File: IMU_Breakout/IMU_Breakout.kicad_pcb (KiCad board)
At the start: 2 copper layers, 12 x 11.2 mm, 4 parts, among them J1 Conn_01x04_Socket, U1 LSM6DSL

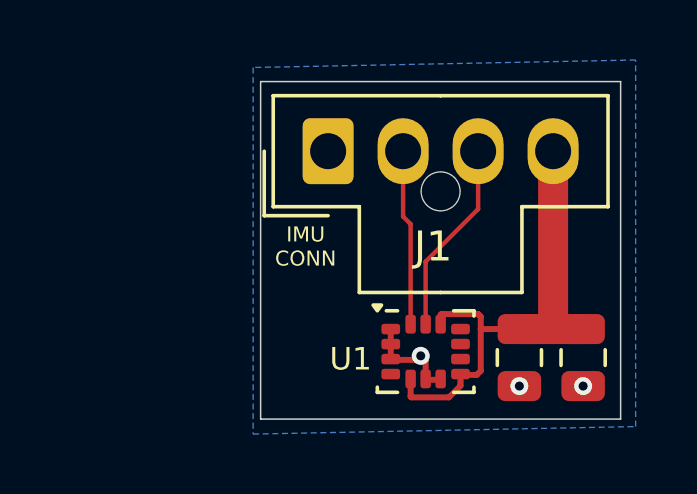
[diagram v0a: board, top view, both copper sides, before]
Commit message: made bom
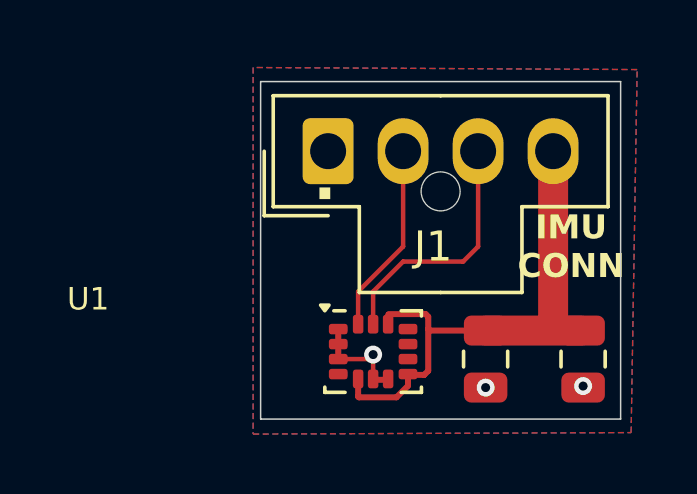
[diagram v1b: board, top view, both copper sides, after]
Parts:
- moved U1 1.75 mm to (146.0, 93.5)
- moved C1 1.13 mm to (149.8, 93.8)
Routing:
- net /IMU_I2C_SCL: track 6.74 -> 8.39 mm
- net +1V8: track 16.5 -> 18.0 mm
- added copper zone on F.Cu, net GND
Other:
- board text added: "."
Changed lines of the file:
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@@
 	(footprint "Capacitor_SMD:C_0805_2012Metric"
 		(layer "F.Cu")
-		(at 150.875 93.7 -90)
+		(at 149.75 93.75 -90)
 		(descr "Capacitor SMD 0805 (2012 Metric), square (rectangular) end terminal, IPC_7351 nominal, (Body size source: IPC-SM-782 page 76, https://www.pcb-3d.com/wordpress/wp-content/uploads/ipc-sm-782a_amendment_1_and_2.pdf, https://docs.google.com/spreadsheets/d/1BsfQQcO9C6DZCsRaXUlFlo91Tg2WpOkGARC1WS5S8t0/edit?usp=sharing), generated with kicad-footprint-generator")
 		(tags "capacitor")
@@
 	(footprint "Capacitor_SMD:C_0805_2012Metric"
 		(layer "F.Cu")
-		(at 153 93.7 -90)
+		(at 153 93.75 -90)
 		(descr "Capacitor SMD 0805 (2012 Metric), square (rectangular) end terminal, IPC_7351 nominal, (Body size source: IPC-SM-782 page 76, https://www.pcb-3d.com/wordpress/wp-content/uploads/ipc-sm-782a_amendment_1_and_2.pdf, https://docs.google.com/spreadsheets/d/1BsfQQcO9C6DZCsRaXUlFlo91Tg2WpOkGARC1WS5S8t0/edit?usp=sharing), generated with kicad-footprint-generator")
 		(tags "capacitor")
@@
 	(footprint "Package_LGA:LGA-14_3x2.5mm_P0.5mm_LayoutBorder3x4y"
 		(layer "F.Cu")
-		(at 147.75 93.5)
+		(at 146 93.5)
 		(descr "LGA, 14 Pin (https://www.st.com/resource/en/datasheet/lsm6ds3tr-c.pdf), generated with kicad-footprint-generator ipc_noLead_generator.py")
 		(tags "LGA NoLead")
 		(property "Reference" "U1"
-			(at -2.5 0.25 0)
+			(at -9.5 -1.75 0)
 			(layer "F.SilkS")
 			(effects
@@
 	)
 	(gr_text "IMU\nCONN"
-		(at 143.75 90 0)
+		(at 152.6 90 0)
 		(layer "F.SilkS")
 		(effects
 			(font
-				(size 0.5 0.5)
-				(thickness 0.125)
-			)
-		)
-	)
-	(segment
-		(start 147.75 92.5875)
-		(end 147.75 90.5)
+				(size 0.8 0.8)
+				(thickness 0.15)
+				(bold yes)
+			)
+		)
+	)
+	(gr_text "."
+		(at 144 88.6 0)
+		(layer "F.SilkS")
+		(effects
+			(font
+				(size 1.5 1.5)
+				(thickness 0.3)
+				(bold yes)
+			)
+			(justify left bottom)
+		)
+	)
+	(segment
+		(start 146 92.5875)
+		(end 146 91.5)
 		(width 0.15)
 		(layer "F.Cu")
@@
 	)
 	(segment
-		(start 149.5 88.75)
-		(end 149.5 86.57)
+		(start 149.5 90)
+		(end 149 90.5)
 		(width 0.15)
 		(layer "F.Cu")
@@
 	)
 	(segment
-		(start 147.75 90.5)
-		(end 149.5 88.75)
+		(start 149.5 86.82)
+		(end 149.5 90)
 		(width 0.15)
 		(layer "F.Cu")
@@
 	)
 	(segment
-		(start 147.25 89.25)
-		(end 147 89)
+		(start 146 91.5)
+		(end 147 90.5)
 		(width 0.15)
 		(layer "F.Cu")
+		(net 1)
+	)
+	(segment
+		(start 147 90.5)
+		(end 149 90.5)
+		(width 0.15)
+		(layer "F.Cu")
+		(net 1)
+	)
+	(segment
+		(start 147 90)
+		(end 147 86.82)
+		(width 0.15)
+		(layer "F.Cu")
 		(net 2)
 	)
 	(segment
-		(start 147.25 92.5875)
-		(end 147.25 89.25)
+		(start 145.5 92.5875)
+		(end 145.5 91.5)
 		(width 0.15)
 		(layer "F.Cu")
@@
 	)
 	(segment
-		(start 147 89)
-		(end 147 86.57)
+		(start 145.5 91.5)
+		(end 147 90)
 		(width 0.15)
 		(layer "F.Cu")
@@
 	)
 	(segment
-		(start 146.5875 93.7775)
-		(end 147.4525 93.7775)
+		(start 146.5 94.44)
+		(end 146 94.44)
 		(width 0.2)
 		(layer "F.Cu")
@@
 	)
 	(segment
-		(start 147.4525 93.7775)
-		(end 147.5875 93.6425)
+		(start 145.85 93.75)
+		(end 146 93.6)
+		(width 0.15)
+		(layer "F.Cu")
+		(net 3)
+	)
+	(segment
+		(start 144.8375 93.75)
+		(end 145.85 93.75)
+		(width 0.15)
+		(layer "F.Cu")
+		(net 3)
+	)
+	(segment
+		(start 146 94.4125)
+		(end 146 93.6)
+		(width 0.15)
+		(layer "F.Cu")
+		(net 3)
+	)
+	(segment
+		(start 144.8375 93.7775)
+		(end 144.8375 92.7775)
 		(width 0.2)
 		(layer "F.Cu")
-		(net 3)
-	)
-	(segment
-		(start 148.25 94.44)
-		(end 147.75 94.44)
-		(width 0.2)
-		(layer "F.Cu")
-		(net 3)
-	)
-	(segment
-		(start 147.75 94.44)
-		(end 147.75 93.805)
-		(width 0.2)
-		(layer "F.Cu")
-		(net 3)
-	)
-	(segment
-		(start 146.5875 93.7775)
-		(end 146.5875 92.7775)
-		(width 0.2)
-		(layer "F.Cu")
-		(net 3)
-	)
-	(segment
-		(start 147.75 93.805)
-		(end 147.5875 93.6425)
-		(width 0.2)
-		(layer "F.Cu")
-		(net 3)
-	)
-	(via
-		(at 147.5875 93.6425)
-		(size 0.6)
-		(drill 0.3)
-		(layers "F.Cu" "B.Cu")
 		(net 3)
 	)
@@
 	)
 	(via
-		(at 150.875 94.65)
+		(at 146 93.6)
+		(size 0.6)
+		(drill 0.3)
+		(layers "F.Cu" "B.Cu")
+		(free yes)
+		(net 3)
+	)
+	(via
+		(at 149.75 94.7)
 		(size 0.6)
 		(drill 0.3)
@@
 	)
 	(segment
-		(start 148.9125 94.2775)
-		(end 149.4525 94.2775)
+		(start 149.75 92.8)
+		(end 152.95 92.8)
+		(width 1)
+		(layer "F.Cu")
+		(net 8)
+	)
+	(segment
+		(start 147.1625 94.2775)
+		(end 147.7025 94.2775)
 		(width 0.2)
 		(layer "F.Cu")
@@
 	)
 	(segment
-		(start 147.25 94.4125)
-		(end 147.25 95)
+		(start 145.5 94.4125)
+		(end 145.5 95)
 		(width 0.2)
 		(layer "F.Cu")
@@
 	)
 	(segment
-		(start 149.5875 94.1425)
-		(end 149.5875 92.75)
+		(start 147.8375 94.1425)
+		(end 147.8375 92.75)
 		(width 0.2)
 		(layer "F.Cu")
@@
 	)
 	(segment
-		(start 152 92.75)
-		(end 150.875 92.75)
-		(width 1)
+		(start 145.5 95)
+		(end 145.525 95.025)
+		(width 0.2)
 		(layer "F.Cu")
 		(net 8)
 	)
 	(segment
-		(start 147.25 95)
-		(end 147.275 95.025)
+		(start 147.8875 92.8)
+		(end 147.8375 92.75)
 		(width 0.2)
 		(layer "F.Cu")
@@
 	)
 	(segment
-		(start 149.5 92.25)
-		(end 148.275001 92.25)
+		(start 147.75 92.25)
+		(end 146.525001 92.25)
 		(width 0.2)
 		(layer "F.Cu")
@@
 	)
 	(segment
-		(start 147.275 95.025)
-		(end 148.527932 95.025)
+		(start 145.525 95.025)
+		(end 146.777932 95.025)
 		(width 0.2)
 		(layer "F.Cu")
@@
 	)
 	(segment
-		(start 148.25 92.275001)
-		(end 148.25 92.5875)
+		(start 149.75 92.8)
+		(end 147.8875 92.8)
 		(width 0.2)
 		(layer "F.Cu")
@@
 	)
 	(segment
-		(start 149.5875 92.75)
-		(end 150.875 92.75)
+		(start 146.5 92.275001)
+		(end 146.5 92.5875)
 		(width 0.2)
 		(layer "F.Cu")
@@
 	)
 	(segment
-		(start 148.527932 95.025)
-		(end 148.9125 94.640432)
+		(start 146.777932 95.025)
+		(end 147.1625 94.640432)
 		(width 0.2)
 		(layer "F.Cu")
@@
 	)
 	(segment
-		(start 149.4525 94.2775)
-		(end 149.5875 94.1425)
+		(start 147.7025 94.2775)
+		(end 147.8375 94.1425)
 		(width 0.2)
 		(layer "F.Cu")
@@
 	)
 	(segment
-		(start 148.9125 94.640432)
-		(end 148.9125 94.2775)
+		(start 147.1625 94.640432)
+		(end 147.1625 94.2775)
 		(width 0.2)
 		(layer "F.Cu")
@@
 	)
 	(segment
-		(start 148.275001 92.25)
-		(end 148.25 92.275001)
+		(start 147.8375 92.75)
+		(end 147.8375 92.3375)
 		(width 0.2)
 		(layer "F.Cu")
@@
 	)
 	(segment
-		(start 149.5875 92.75)
-		(end 149.5875 92.3375)
+		(start 147.8375 92.3375)
+		(end 147.75 92.25)
 		(width 0.2)
-		(layer "F.Cu")
-		(net 8)
-	)
-	(segment
-		(start 149.5875 92.3375)
-		(end 149.5 92.25)
-		(width 0.2)
-		(layer "F.Cu")
-		(net 8)
-	)
-	(segment
-		(start 153.125 92.75)
-		(end 152 92.75)
-		(width 1)
 		(layer "F.Cu")
 		(net 8)
@@
 		(net 3)
 		(net_name "GND")
-		(layer "B.Cu")
+		(layers "F&B.Cu")
 		(hatch edge 0.5)
 		(connect_pads
@@
 		(polygon
 			(pts
-				(xy 142 84.030762) (xy 142 96.25) (xy 154.75 96) (xy 154.75 83.780762)
-			)
-		)
+				(xy 142 84.030762) (xy 142 96.25) (xy 154.6 96.2) (xy 154.8 84.1)
+			)
+		)
